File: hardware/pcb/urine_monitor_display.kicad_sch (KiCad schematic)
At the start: 1 part, among them J2 EInk_FPC

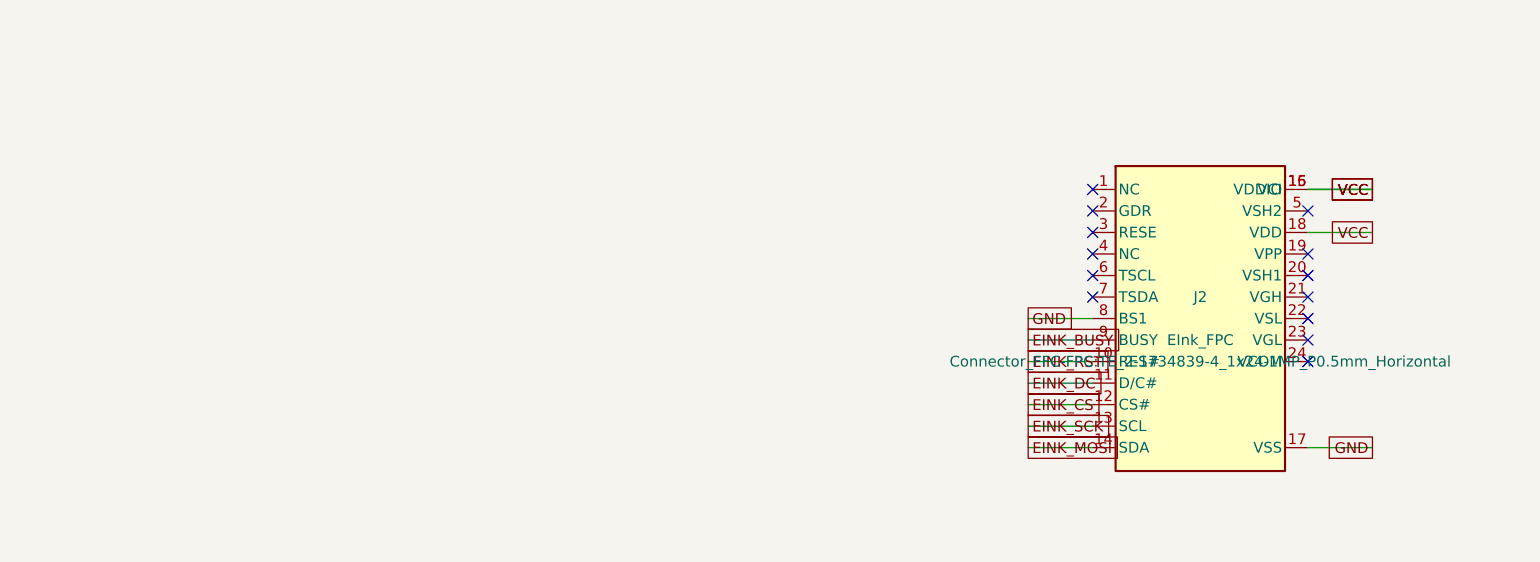
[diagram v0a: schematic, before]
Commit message: init
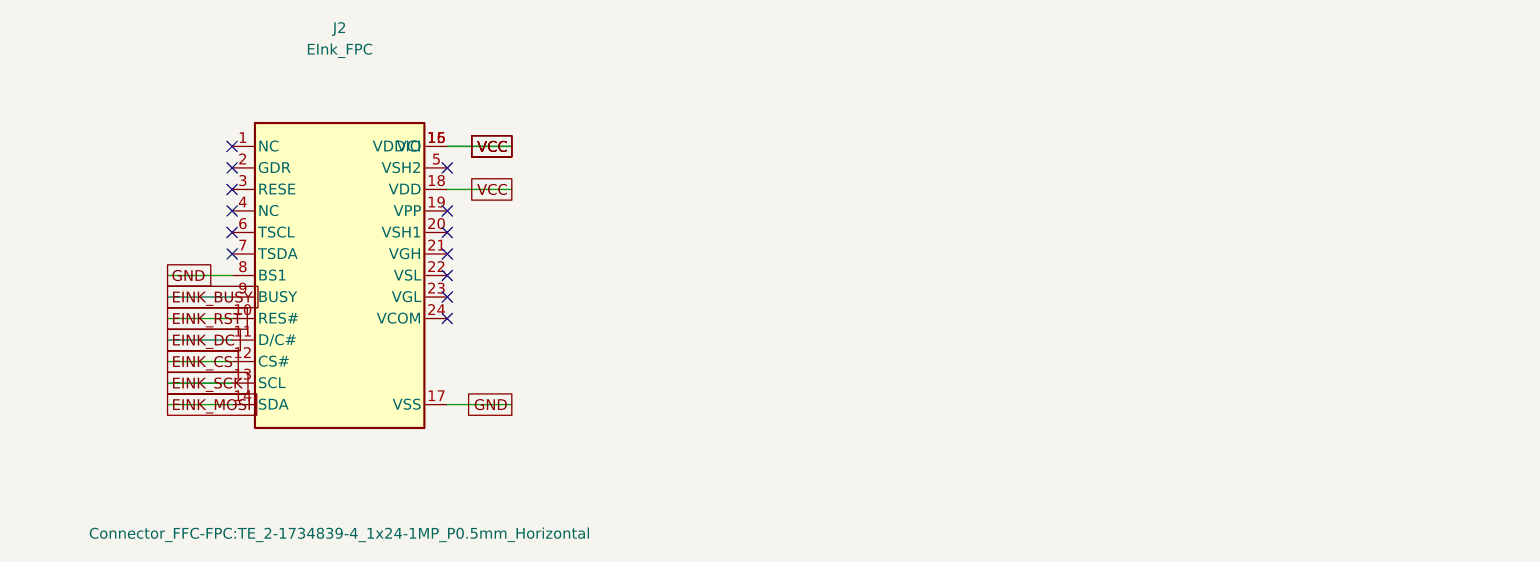
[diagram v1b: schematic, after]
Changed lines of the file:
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@@
     (title "E-Ink Display")
   )
-  (symbol (lib_id "Project_Lib:GDEY0213B74") (at 250.19 110.49 0) (unit 1)
+  (symbol (lib_id "Project_Lib:GDEY0213B74") (at 148.59 105.41 0) (unit 1)
     (in_bom yes) (on_board yes)
-    (property "Reference" "J2" (id 0) (at 250.19 107.95 0)
-      (effects (font (size 1.27 1.27)))
+    (property "Reference" "J2" (id 0) (at 148.59 76.20 0)
+      (effects (font (size 1.27 1.27)) (justify center))
     )
-    (property "Value" "EInk_FPC" (id 1) (at 250.19 113.03 0)
-      (effects (font (size 1.27 1.27)))
+    (property "Value" "EInk_FPC" (id 1) (at 148.59 78.74 0)
+      (effects (font (size 1.27 1.27)) (justify center))
     )
-    (property "Footprint" "Connector_FFC-FPC:TE_2-1734839-4_1x24-1MP_P0.5mm_Horizontal" (id 2) (at 250.19 115.57 0) (effects (font (size 1.27 1.27))))
+    (property "Footprint" "Connector_FFC-FPC:TE_2-1734839-4_1x24-1MP_P0.5mm_Horizontal" (id 2) (at 148.59 135.89 0) (effects (font (size 1.27 1.27)) (justify center)))
   )
   (symbol_instances
-    (path "/839e2451-f023-487b-83ca-a3957f7538dd/5df45be0-fc22-464e-8282-79889db5c0fd" (reference "J2") (unit 1))
+    (path "/30e59c9d-3e12-4723-8c15-c145e7d3c8ac/2ee36964-4a77-474c-bb52-1b699e6d7e61" (reference "J2") (unit 1))
   )
-  (wire (pts (xy 237.49 113.03) (xy 229.87 113.03)))
-  (global_label "EINK_BUSY" (shape passive) (at 229.87 113.03 0) (effects (font (size 1.27 1.27)) (justify left)))
-  (wire (pts (xy 237.49 120.65) (xy 229.87 120.65)))
-  (global_label "EINK_CS" (shape passive) (at 229.87 120.65 0) (effects (font (size 1.27 1.27)) (justify left)))
-  (wire (pts (xy 237.49 118.11) (xy 229.87 118.11)))
-  (global_label "EINK_DC" (shape passive) (at 229.87 118.11 0) (effects (font (size 1.27 1.27)) (justify left)))
-  (wire (pts (xy 237.49 125.73) (xy 229.87 125.73)))
-  (global_label "EINK_MOSI" (shape passive) (at 229.87 125.73 0) (effects (font (size 1.27 1.27)) (justify left)))
-  (wire (pts (xy 237.49 115.57) (xy 229.87 115.57)))
-  (global_label "EINK_RST" (shape passive) (at 229.87 115.57 0) (effects (font (size 1.27 1.27)) (justify left)))
-  (wire (pts (xy 237.49 123.19) (xy 229.87 123.19)))
-  (global_label "EINK_SCK" (shape passive) (at 229.87 123.19 0) (effects (font (size 1.27 1.27)) (justify left)))
-  (wire (pts (xy 262.89 125.73) (xy 270.51 125.73)))
-  (global_label "GND" (shape passive) (at 270.51 125.73 0) (effects (font (size 1.27 1.27)) (justify right)))
-  (wire (pts (xy 237.49 110.49) (xy 229.87 110.49)))
-  (global_label "GND" (shape passive) (at 229.87 110.49 0) (effects (font (size 1.27 1.27)) (justify left)))
-  (wire (pts (xy 262.89 95.25) (xy 270.51 95.25)))
-  (global_label "VCC" (shape passive) (at 270.51 95.25 0) (effects (font (size 1.27 1.27)) (justify right)))
-  (wire (pts (xy 262.89 95.25) (xy 270.51 95.25)))
-  (global_label "VCC" (shape passive) (at 270.51 95.25 0) (effects (font (size 1.27 1.27)) (justify right)))
-  (wire (pts (xy 262.89 100.33) (xy 270.51 100.33)))
-  (global_label "VCC" (shape passive) (at 270.51 100.33 0) (effects (font (size 1.27 1.27)) (justify right)))
-  (no_connect (at 237.49 95.25))
-  (no_connect (at 237.49 97.79))
-  (no_connect (at 237.49 100.33))
-  (no_connect (at 237.49 102.87))
-  (no_connect (at 262.89 97.79))
-  (no_connect (at 237.49 105.41))
-  (no_connect (at 237.49 107.95))
-  (no_connect (at 262.89 102.87))
-  (no_connect (at 262.89 105.41))
-  (no_connect (at 262.89 107.95))
-  (no_connect (at 262.89 110.49))
-  (no_connect (at 262.89 113.03))
-  (no_connect (at 262.89 115.57))
+  (wire (pts (xy 135.89 107.95) (xy 128.27 107.95)))
+  (global_label "EINK_BUSY" (shape passive) (at 128.27 107.95 0) (effects (font (size 1.27 1.27)) (justify left)))
+  (wire (pts (xy 135.89 115.57) (xy 128.27 115.57)))
+  (global_label "EINK_CS" (shape passive) (at 128.27 115.57 0) (effects (font (size 1.27 1.27)) (justify left)))
+  (wire (pts (xy 135.89 113.03) (xy 128.27 113.03)))
+  (global_label "EINK_DC" (shape passive) (at 128.27 113.03 0) (effects (font (size 1.27 1.27)) (justify left)))
+  (wire (pts (xy 135.89 120.65) (xy 128.27 120.65)))
+  (global_label "EINK_MOSI" (shape passive) (at 128.27 120.65 0) (effects (font (size 1.27 1.27)) (justify left)))
+  (wire (pts (xy 135.89 110.49) (xy 128.27 110.49)))
+  (global_label "EINK_RST" (shape passive) (at 128.27 110.49 0) (effects (font (size 1.27 1.27)) (justify left)))
+  (wire (pts (xy 135.89 118.11) (xy 128.27 118.11)))
+  (global_label "EINK_SCK" (shape passive) (at 128.27 118.11 0) (effects (font (size 1.27 1.27)) (justify left)))
+  (wire (pts (xy 161.29 120.65) (xy 168.91 120.65)))
+  (global_label "GND" (shape passive) (at 168.91 120.65 0) (effects (font (size 1.27 1.27)) (justify right)))
+  (wire (pts (xy 135.89 105.41) (xy 128.27 105.41)))
+  (global_label "GND" (shape passive) (at 128.27 105.41 0) (effects (font (size 1.27 1.27)) (justify left)))
+  (wire (pts (xy 161.29 90.17) (xy 168.91 90.17)))
+  (global_label "VCC" (shape passive) (at 168.91 90.17 0) (effects (font (size 1.27 1.27)) (justify right)))
+  (wire (pts (xy 161.29 90.17) (xy 168.91 90.17)))
+  (global_label "VCC" (shape passive) (at 168.91 90.17 0) (effects (font (size 1.27 1.27)) (justify right)))
+  (wire (pts (xy 161.29 95.25) (xy 168.91 95.25)))
+  (global_label "VCC" (shape passive) (at 168.91 95.25 0) (effects (font (size 1.27 1.27)) (justify right)))
+  (no_connect (at 135.89 90.17))
+  (no_connect (at 135.89 92.71))
+  (no_connect (at 135.89 95.25))
+  (no_connect (at 135.89 97.79))
+  (no_connect (at 161.29 92.71))
+  (no_connect (at 135.89 100.33))
+  (no_connect (at 135.89 102.87))
+  (no_connect (at 161.29 97.79))
+  (no_connect (at 161.29 100.33))
+  (no_connect (at 161.29 102.87))
+  (no_connect (at 161.29 105.41))
+  (no_connect (at 161.29 107.95))
+  (no_connect (at 161.29 110.49))
   (sheet_instances
-    (path "/839e2451-f023-487b-83ca-a3957f7538dd/5df45be0-fc22-464e-8282-79889db5c0fd" (page "5"))
+    (path "/30e59c9d-3e12-4723-8c15-c145e7d3c8ac/2ee36964-4a77-474c-bb52-1b699e6d7e61" (page "5"))
   )
   (embedded_fonts no)
